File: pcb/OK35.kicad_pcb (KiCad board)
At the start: 2 copper layers, 133.3 x 116.2 mm, 81 parts, among them SW1 SW_SPST, SW10 SW_SPST, SW11 SW_SPST, SW12 SW_SPST, SW13 SW_SPST, SW14 SW_SPST, SW15 SW_SPST, SW16 SW_SPST, SW17 SW_SPST, SW18 SW_SPST, SW19 SW_SPST, SW2 SW_SPST, SW20 SW_SPST, SW21 SW_SPST, SW22 SW_SPST, SW23 SW_SPST, SW24 SW_SPST, SW25 SW_SPST, SW26 SW_SPST, SW27 SW_SPST, SW28 SW_SPST, SW29 SW_SPST, SW3 SW_SPST, SW30 SW_SPST, SW31 SW_SPST, SW32 SW_SPST, SW33 SW_SPST, SW34 SW_SPST, SW35 SW_SPST, SW36 SW_SPST, SW37 SW_SPST, SW4 SW_SPST, SW5 SW_SPST, SW6 SW_SPST, SW7 SW_SPST, SW8 SW_SPST, SW9 SW_SPST, U1 TRRS, U2 ProMicro

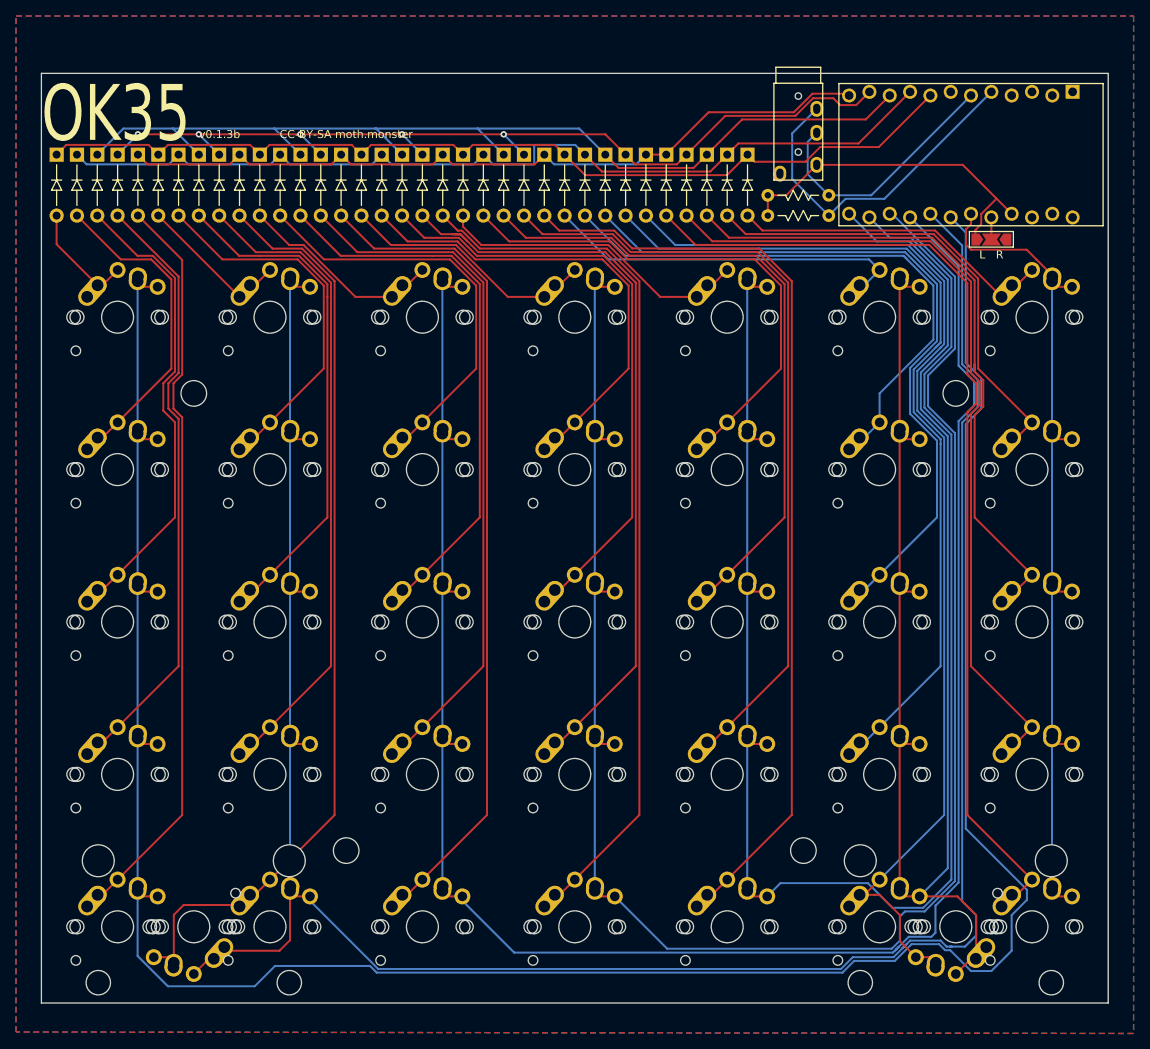
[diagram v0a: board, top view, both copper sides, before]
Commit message: Revert "v0.1.3b - moved some holes"
This reverts commit e650355a7cdd176761959e97b09434696344432b.
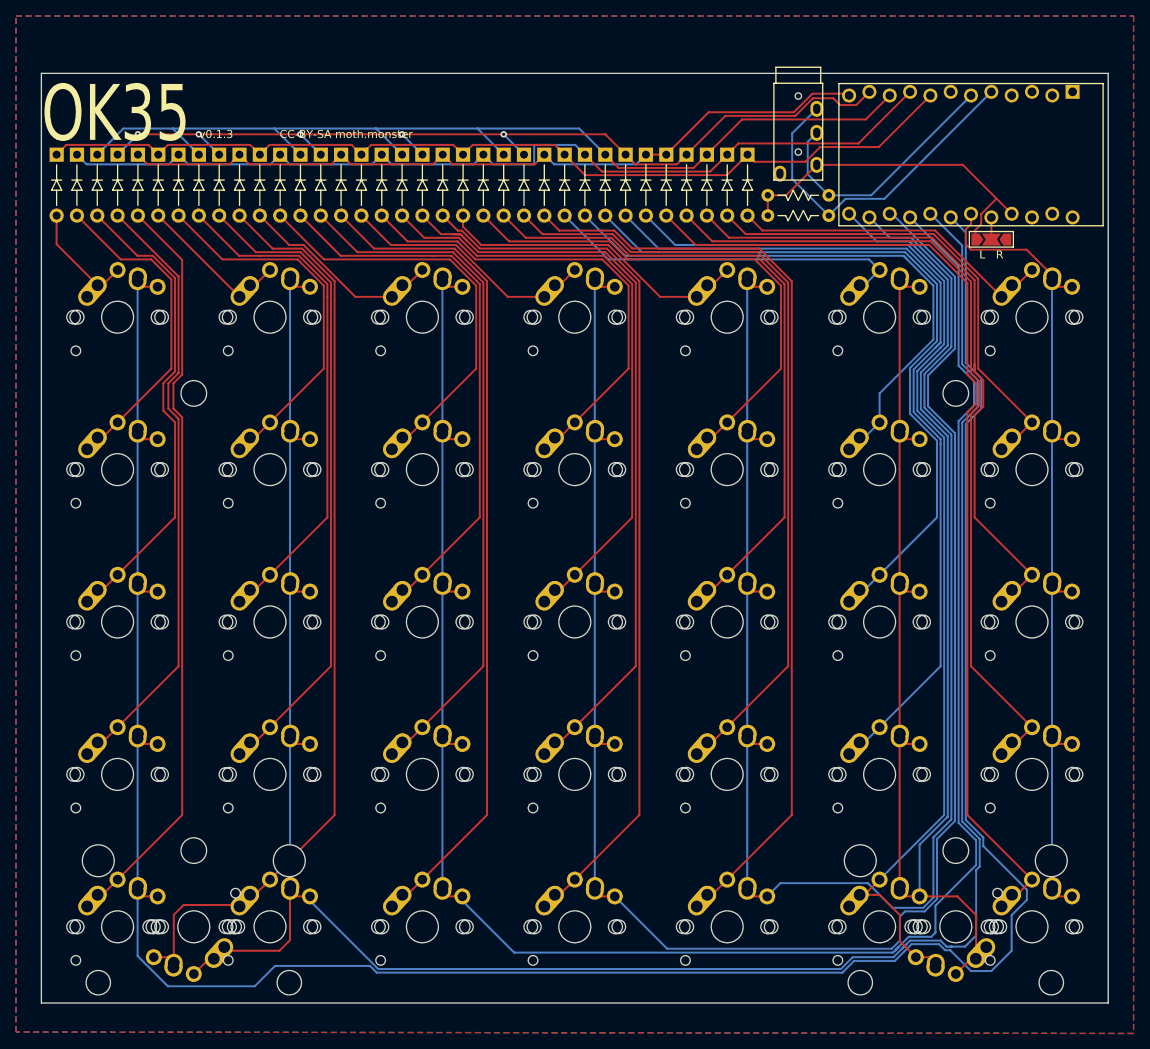
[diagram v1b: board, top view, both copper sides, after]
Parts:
- moved REF** 19.1 mm to (193.7, 129.7)
- moved REF** 19.0 mm to (98.4, 129.7)
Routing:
- net Col2: track 248.9 -> 250.7 mm
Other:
- board text added: "v0.1.3"
- board text removed: "v0.1.3b"

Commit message: v0.1.3b - moved some holes
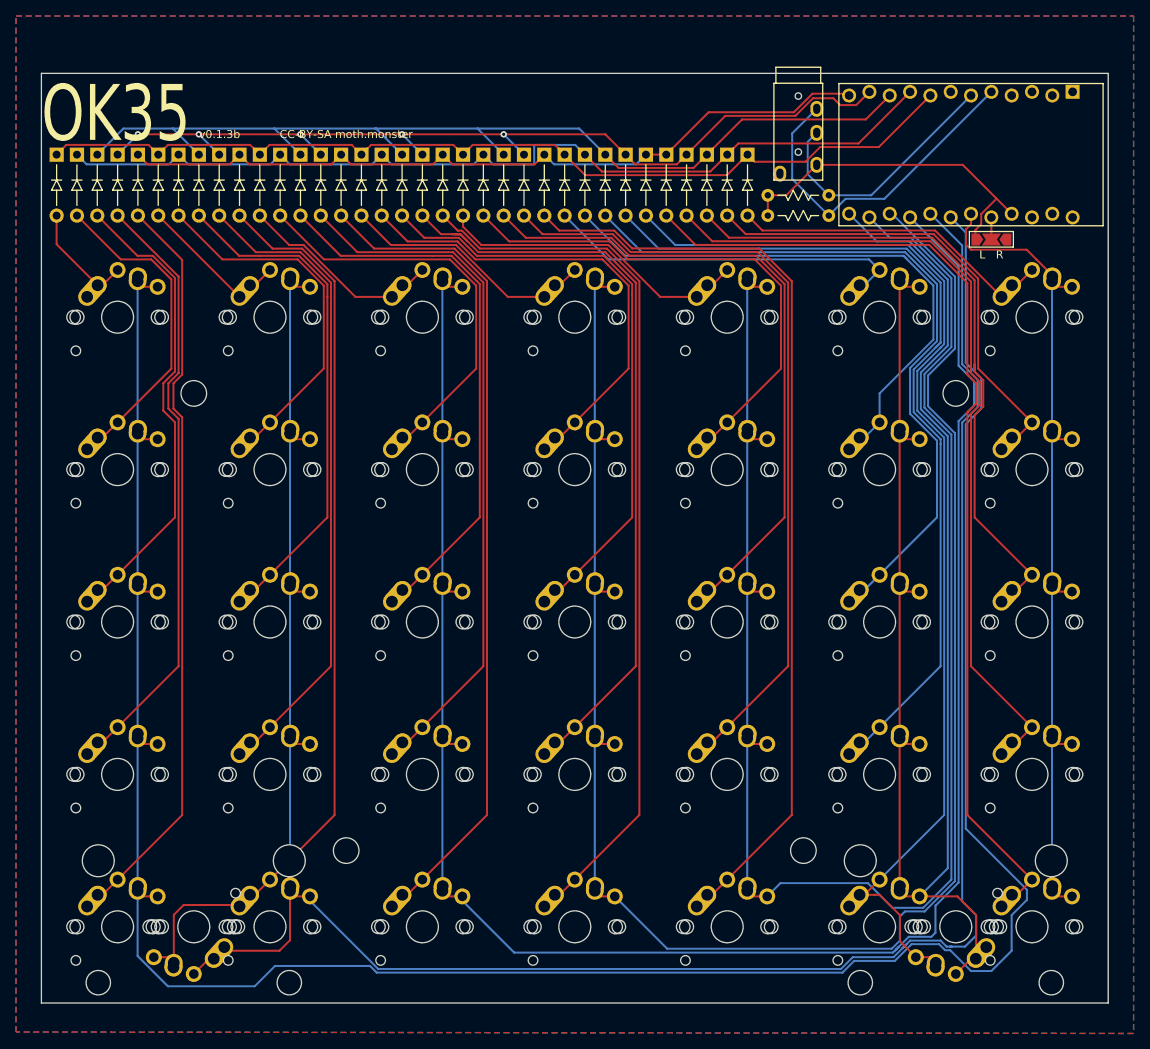
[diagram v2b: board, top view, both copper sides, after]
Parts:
- moved REF** 19.1 mm to (174.6, 129.7)
- moved REF** 19.0 mm to (117.5, 129.7)
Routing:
- net Col2: track 250.7 -> 248.9 mm
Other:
- board text added: "v0.1.3b"
- board text removed: "v0.1.3"
